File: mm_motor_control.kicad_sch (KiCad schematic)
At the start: 0 parts

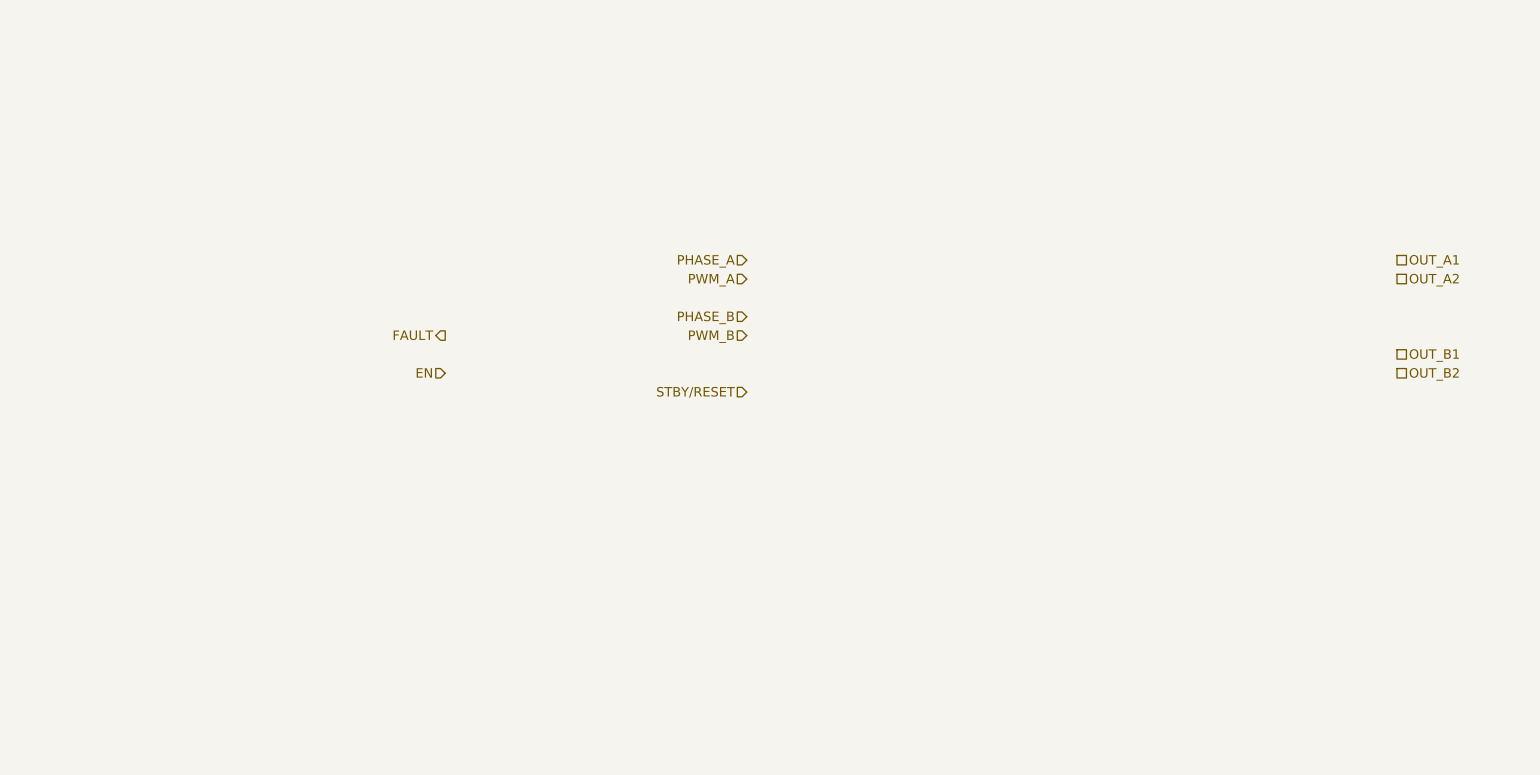
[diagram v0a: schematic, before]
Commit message: fin tp2
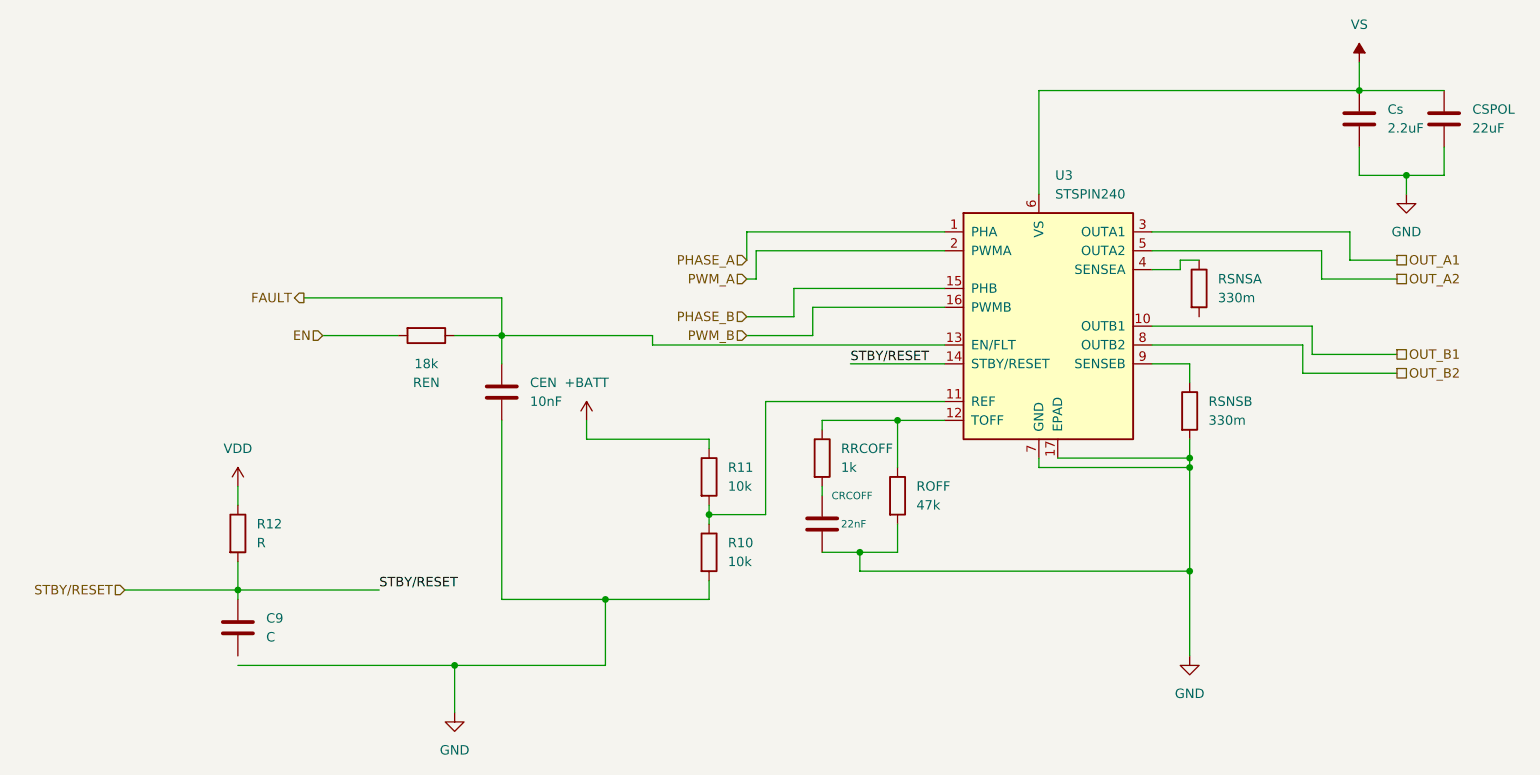
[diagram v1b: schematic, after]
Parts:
- added C9: C, symbol Device:C
- added CEN: 10nF, symbol Device:C
- added CRCOFF: 22nF, symbol Device:C
- added CSPOL: 22uF, symbol Device:C
- added Cs: 2.2uF, symbol Device:C
- added R10, R11: 10k, symbol Device:R
- added R12: R, symbol Device:R
- added REN: 18k, symbol Device:R
- added ROFF: 47k, symbol Device:R
- added RRCOFF: 1k, symbol Device:R
- added RSNSA, RSNSB: 330m, symbol Device:R
- added U3: STSPIN240, Package_DFN_QFN:VQFN-16-1EP_3x3mm_P0.5mm_EP1.8x1.8mm, symbol Driver_Motor:STSPIN240
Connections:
- net EN: now also REN.2
- net FAULT: now also CEN.1, REN.1, U3.13 (EN/FLT)
- net OUT_A1: now also U3.3 (OUTA1)
- net OUT_A2: now also U3.5 (OUTA2)
- net OUT_B1: now also U3.10 (OUTB1)
- net OUT_B2: now also U3.8 (OUTB2)
- net PHASE_A: now also U3.1 (PHA)
- net PHASE_B: now also U3.15 (PHB)
- net PWM_A: now also U3.2 (PWMA)
- net PWM_B: now also U3.16 (PWMB)
- net STBY/RESET: now also C9.1, R12.2, U3.14 (STBY/RESET)
- new net: ROFF.1, RRCOFF.1, U3.12 (TOFF)
- new net: CRCOFF.1, RRCOFF.2
- new net: R10.1, R11.2, U3.11 (REF)
- new net: RSNSA.1, U3.4 (SENSEA)
- new net: RSNSB.1, U3.9 (SENSEB)
- new net +BATT: R11.1
- new net GND: CEN.2, CRCOFF.2, CSPOL.2, Cs.2, R10.2, ROFF.2, RSNSB.2, U3.17 (EPAD), U3.7 (GND)
- new net VDD: R12.1
- new net VS: CSPOL.1, Cs.1, U3.6 (VS)
